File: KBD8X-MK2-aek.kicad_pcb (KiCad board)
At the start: 2 copper layers, 343.7 x 118.3 mm, 215 parts, among them J1 AVR-ISP-6, Q1 DSS60601MZ4-13, SW1 SW_Push, U1 ATmega32U4-MU, U2 PRTR5V0U2X, Y1 16MHz

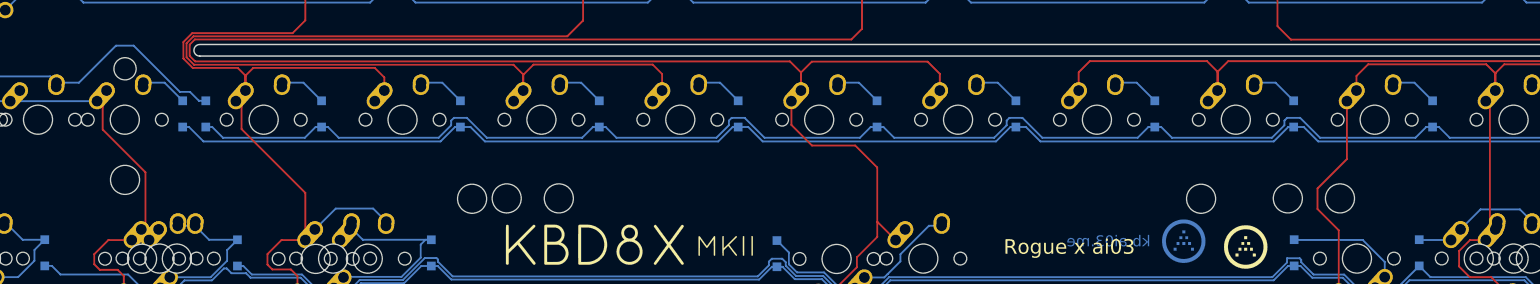
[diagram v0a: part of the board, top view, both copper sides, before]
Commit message: cleanup
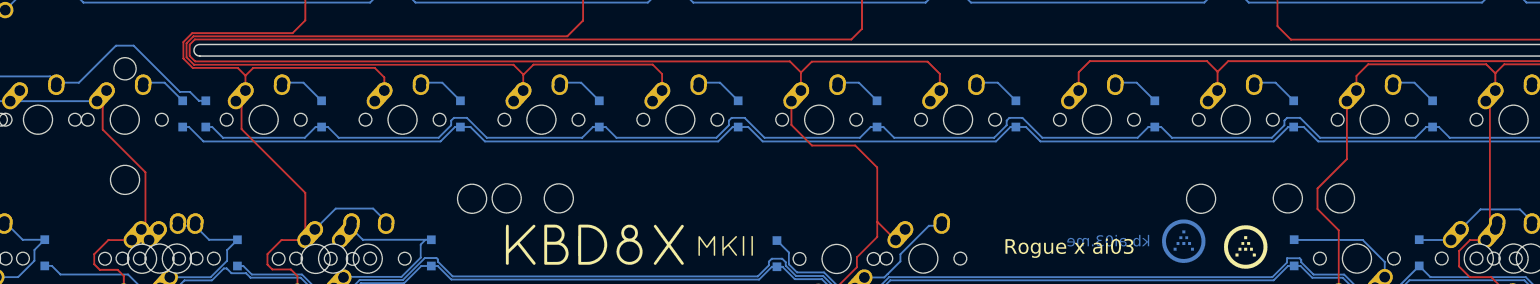
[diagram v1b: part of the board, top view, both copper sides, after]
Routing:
- net COL4: track 431.8 -> 429.3 mm
- net COL3: track 618.0 -> 615.6 mm
- net COL5: track 351.7 -> 349.3 mm
- net COL2: track 415.2 -> 413.0 mm
- net COL1: track 312.6 -> 310.5 mm
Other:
- outline, holes or cut-outs redrawn
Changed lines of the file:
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@@
     (fp_line (start -2.35 1.15) (end -2.35 -1.15) (layer "B.CrtYd") (width 0.05))
     (fp_line (start -2.35 1.15) (end 2.35 1.15) (layer "B.CrtYd") (width 0.05))
+    (fp_line (start 0.25 0.4) (end 0.25 -0.4) (layer "B.Fab") (width 0.1))
+    (fp_line (start -0.35 0) (end -0.35 -0.55) (layer "B.Fab") (width 0.1))
+    (fp_line (start -1.4 0.9) (end 1.4 0.9) (layer "B.Fab") (width 0.1))
+    (fp_line (start -0.35 0) (end -0.35 0.55) (layer "B.Fab") (width 0.1))
     (fp_line (start 0.25 0) (end 0.75 0) (layer "B.Fab") (width 0.1))
-    (fp_line (start 0.25 0.4) (end 0.25 -0.4) (layer "B.Fab") (width 0.1))
+    (fp_line (start -0.75 0) (end -0.35 0) (layer "B.Fab") (width 0.1))
     (fp_line (start 1.4 0.9) (end 1.4 -0.9) (layer "B.Fab") (width 0.1))
-    (fp_line (start -0.35 0) (end -0.35 -0.55) (layer "B.Fab") (width 0.1))
+    (fp_line (start 0.25 -0.4) (end -0.35 0) (layer "B.Fab") (width 0.1))
     (fp_line (start 1.4 -0.9) (end -1.4 -0.9) (layer "B.Fab") (width 0.1))
-    (fp_line (start -1.4 0.9) (end 1.4 0.9) (layer "B.Fab") (width 0.1))
     (fp_line (start -1.4 -0.9) (end -1.4 0.9) (layer "B.Fab") (width 0.1))
-    (fp_line (start 0.25 -0.4) (end -0.35 0) (layer "B.Fab") (width 0.1))
-    (fp_line (start -0.75 0) (end -0.35 0) (layer "B.Fab") (width 0.1))
-    (fp_line (start -0.35 0) (end -0.35 0.55) (layer "B.Fab") (width 0.1))
     (fp_line (start -0.35 0) (end 0.25 0.4) (layer "B.Fab") (width 0.1))
     (pad "1" smd rect locked (at -1.8 0 90) (size 1.2 1.2) (layers "B.Cu" "B.Paste" "B.Mask")
@@
   (gr_line (start 43.259375 31.75) (end 320.278125 31.75) (layer "Edge.Cuts") (width 0.2))
   (gr_arc (start 67.46875 73.81875) (mid 66.675 73.025) (end 67.46875 72.23125) (layer "Edge.Cuts") (width 0.2))
-  (gr_arc (start 81.715592 111.925733) (mid 80.921842 111.131983) (end 81.715592 110.338233) (layer "Edge.Cuts") (width 0.2))
+  (gr_arc (start 81.720503 111.918093) (mid 80.926753 111.124343) (end 81.720503 110.330593) (layer "Edge.Cuts") (width 0.2))
   (gr_arc (start 321.071875 30.95625) (mid 320.839391 31.517516) (end 320.278125 31.75) (layer "Edge.Cuts") (width 0.2))
   (gr_arc (start 380.603125 31.75) (mid 382.848189 32.679936) (end 383.778125 34.925) (layer "Edge.Cuts") (width 0.2))
@@
   (segment (start 52.667799 143.752547) (end 54.175418 142.244928) (width 0.254) (layer "B.Cu") (net 81))
   (segment (start 54.9275 134.62) (end 57.426594 137.119094) (width 0.254) (layer "B.Cu") (net 81))
-  (segment (start 60.445297 137.119094) (end 60.458141 137.10625) (width 0.254) (layer "B.Cu") (net 81))
   (segment (start 86.886458 137.114749) (end 82.992662 137.114749) (width 0.254) (layer "B.Cu") (net 82))
   (segment (start 85.471799 138.540272) (end 85.471799 140.003869) (width 0.254) (layer "B.Cu") (net 82))
@@
   (segment (start 134.3025 107.052148) (end 132.140902 109.213746) (width 0.254) (layer "F.Cu") (net 100))
   (segment (start 134.3025 99.06) (end 134.3025 97.4725) (width 0.254) (layer "F.Cu") (net 100))
-  (segment (start 126.0875 116.65) (end 126.0875 114.504975) (width 0.254) (layer "F.Cu") (net 100))
   (segment (start 124.754176 113.11088) (end 126.0875 114.444204) (width 0.254) (layer "F.Cu") (net 100))
   (segment (start 134.3025 97.4725) (end 130.175 93.345) (width 0.254) (layer "F.Cu") (net 100))
@@
   (segment (start 94.446387 108.782426) (end 80.685074 108.782427) (width 0.254) (layer "F.Cu") (net 101))
   (segment (start 82.55 37.7825) (end 82.55 60.325) (width 0.254) (layer "F.Cu") (net 101))
-  (segment (start 87.9875 116.65) (end 87.9875 114.619984) (width 0.254) (layer "F.Cu") (net 101))
   (segment (start 92.931776 137.16) (end 91.007132 139.084644) (width 0.254) (layer "F.Cu") (net 101))
   (segment (start 92.075 93.218) (end 92.075 80.645) (width 0.254) (layer "F.Cu") (net 101))
@@
   (segment (start 177.8 61.595) (end 177.165 60.96) (width 0.254) (layer "F.Cu") (net 102))
   (segment (start 168.508051 144.250951) (end 171.864828 140.894174) (width 0.254) (layer "F.Cu") (net 102))
-  (segment (start 164.1875 116.65) (end 164.1875 114.178214) (width 0.254) (layer "F.Cu") (net 102))
   (segment (start 65.786 72.009) (end 65.786 74.041) (width 0.254) (layer "F.Cu") (net 102))
   (segment (start 81.042392 109.645065) (end 80.338876 110.348581) (width 0.254) (layer "F.Cu") (net 102))
@@
   (segment (start 229.5525 99.06) (end 229.5525 97.4725) (width 0.254) (layer "F.Cu") (net 103))
   (segment (start 210.5025 97.4725) (end 206.375 93.345) (width 0.254) (layer "F.Cu") (net 103))
-  (segment (start 221.3375 114.074469) (end 221.3375 116.65) (width 0.254) (layer "F.Cu") (net 103))
   (segment (start 213.487 71.374) (end 199.39 71.374) (width 0.254) (layer "F.Cu") (net 103))
   (segment (start 286.639 72.009) (end 286.004 71.374) (width 0.254) (layer "F.Cu") (net 103))
@@
   (segment (start 256.032 70.866) (end 254 68.834) (width 0.254) (layer "F.Cu") (net 104))
   (segment (start 255.968669 137.16) (end 254.46775 138.660919) (width 0.254) (layer "F.Cu") (net 104))
-  (segment (start 259.4375 116.65) (end 259.4375 114.295501) (width 0.254) (layer "F.Cu") (net 104))
   (segment (start 244.475 80.645) (end 243.84 80.01) (width 0.254) (layer "F.Cu") (net 104))
   (segment (start 248.6025 99.06) (end 248.6025 97.4725) (width 0.254) (layer "F.Cu") (net 104))
